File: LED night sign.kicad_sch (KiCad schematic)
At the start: 38 parts, among them Q1 MOSFET-NCH-2N7002PW, Q2 BC817, U1 ATtiny85-20M, U2 APDS-9301

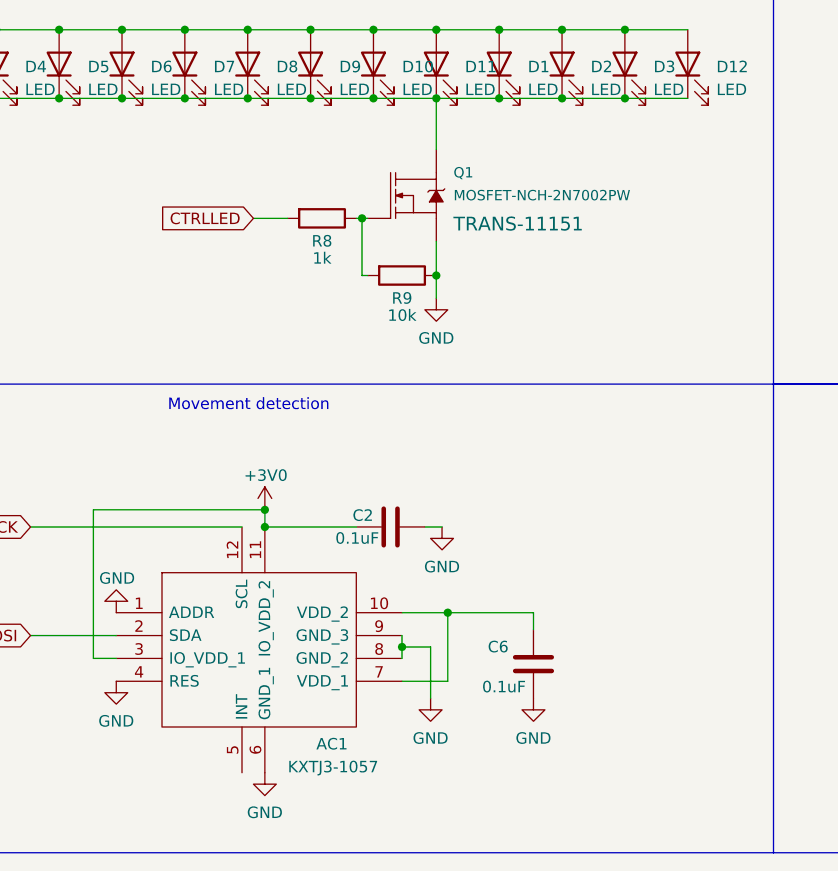
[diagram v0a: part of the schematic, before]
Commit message: enh schematic and added pdf
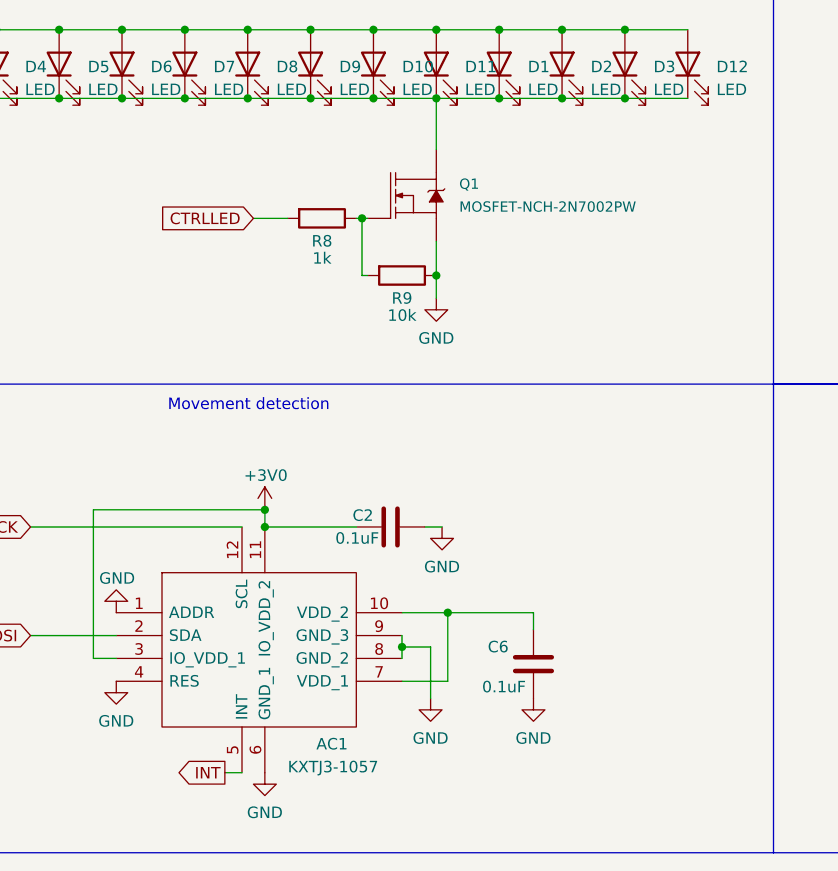
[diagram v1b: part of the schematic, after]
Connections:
- net INT: now also AC1.5 (INT)
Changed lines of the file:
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@@
+    (stroke (width 0) (type default) (color 0 0 0 0))
+  )
+  (wire (pts (xy 61.595 112.395) (xy 63.5 112.395))
     (stroke (width 0) (type default) (color 0 0 0 0))
   )
@@
     (property "Intersheet References" "${INTERSHEET_REFS}" (id 0) (at 201.531 34.8456 0)
       (effects (font (size 1.27 1.27)) (justify left) hide)
+    )
+  )
+  (global_label "INT" (shape output) (at 61.595 112.395 180) (fields_autoplaced)
+    (effects (font (size 1.27 1.27)) (justify right))
+    (property "Intersheet References" "${INTERSHEET_REFS}" (id 0) (at 56.279 112.3156 0)
+      (effects (font (size 1.27 1.27)) (justify right) hide)
     )
   )
@@
   (symbol (lib_id "SparkFun-DiscreteSemi:MOSFET-NCH-2N7002PW") (at 82.55 48.26 0) (unit 1)
     (in_bom yes) (on_board yes) (fields_autoplaced)
-    (property "Reference" "Q1" (id 0) (at 86.995 45.72 0)
+    (property "Reference" "Q1" (id 0) (at 87.63 46.99 0)
       (effects (font (size 1.143 1.143)) (justify left))
     )
-    (property "Value" "MOSFET-NCH-2N7002PW" (id 1) (at 86.995 48.26 0)
+    (property "Value" "MOSFET-NCH-2N7002PW" (id 1) (at 87.63 49.53 0)
       (effects (font (size 1.143 1.143)) (justify left))
     )
@@
     )
     (property "Field4" "TRANS-11151" (id 4) (at 86.995 51.435 0)
-      (effects (font (size 1.524 1.524)) (justify left))
-    )
-    (pin "1")
+      (effects (font (size 1.524 1.524)) (justify left) hide)
+    )
+    (pin "1")
